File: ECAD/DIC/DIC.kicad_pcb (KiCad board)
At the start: 4 copper layers, 68.1 x 55.2 mm, 113 parts, among them J1 WE 62702621621, Q1 BC846, Q2 BC846, Q3 BC846, Q4 BC846, Q5 BC846, Q6 BC846, Q7 BC846, Q8 BC846, U1 R-78E5.0-1.0, U10 ADA4500-2, U2 MCP130-270, U3 STM32F072RBTx, U5 R-78E3.3-1.0, U7 MCP2562-E-SN, U8 NCP1117-12, U9 ADA4500-2, Y1 WE830055951

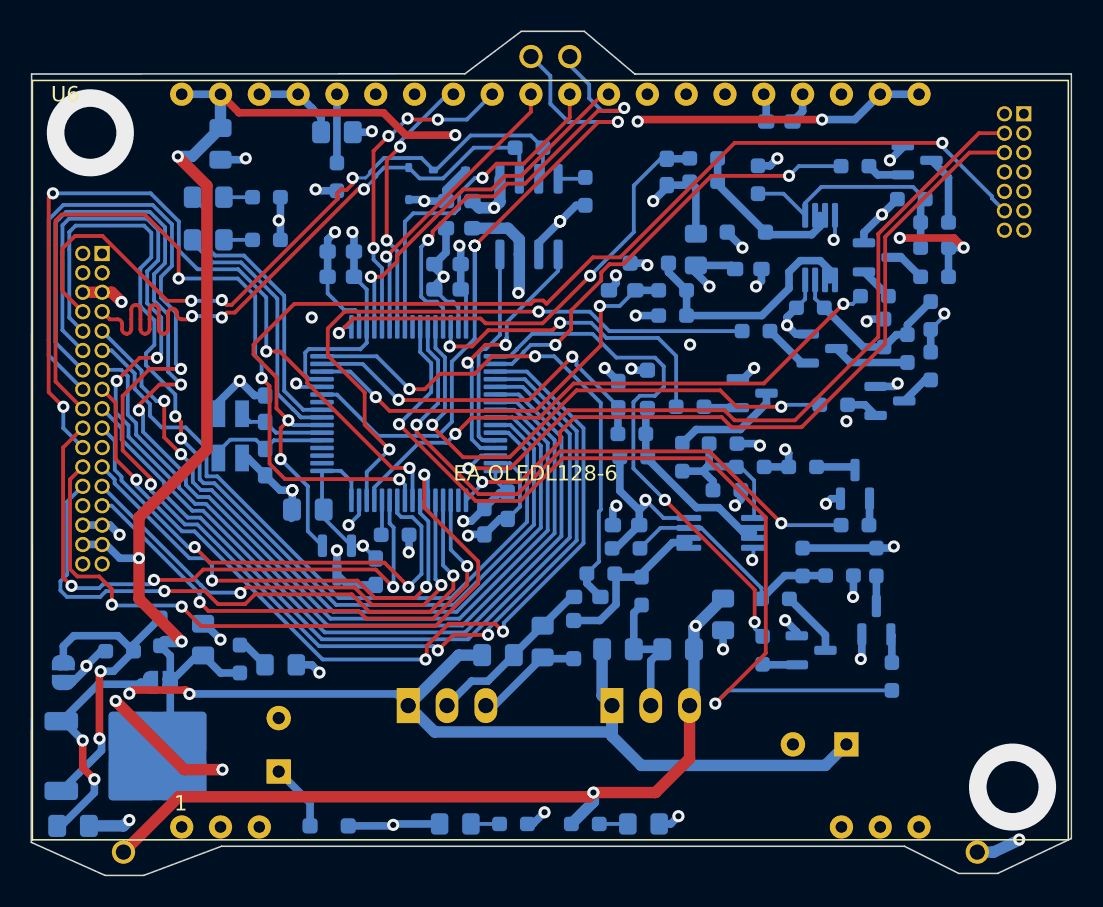
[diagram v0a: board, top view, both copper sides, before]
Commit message: finisjed PCB projekt
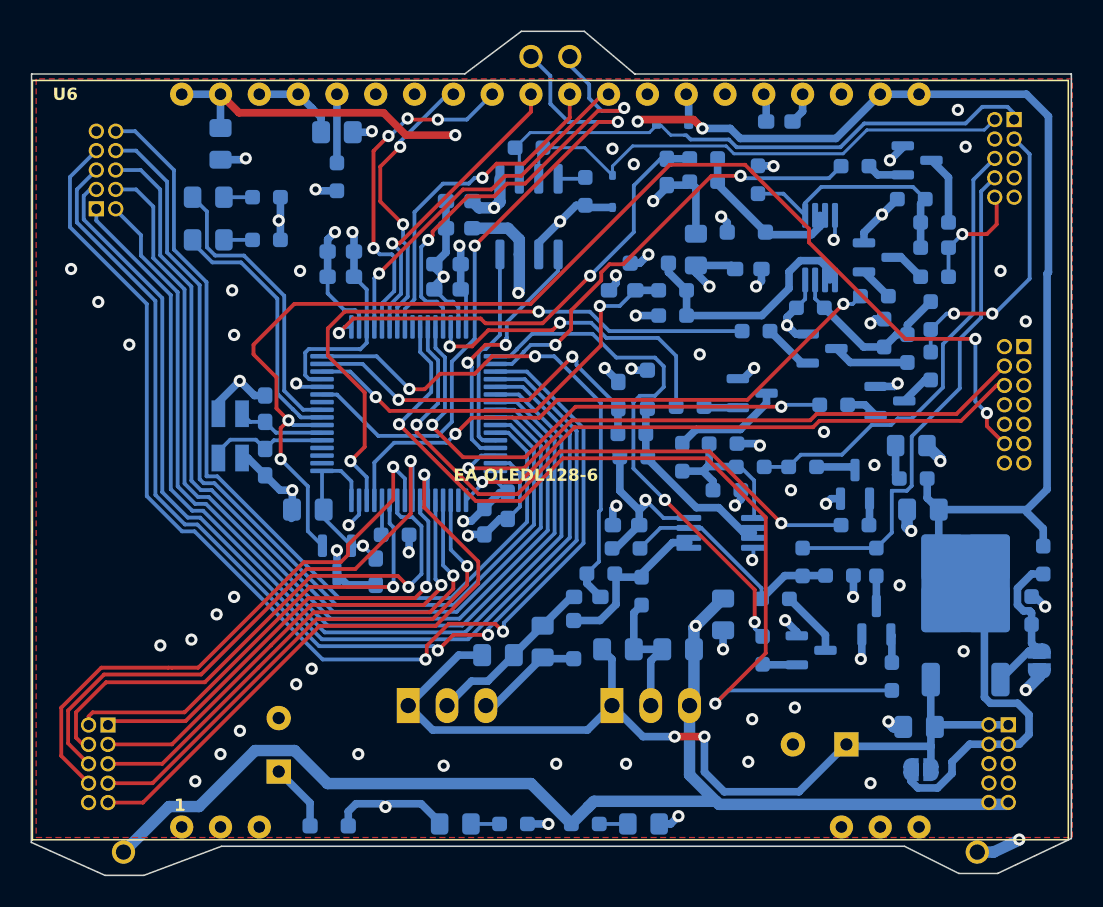
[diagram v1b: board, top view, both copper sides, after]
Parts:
- removed J1: WE 62702621621, Connector_PinHeader_1.27mm:PinHeader_2x17_P1.27mm_Vertical
- added J2: Conn_02x05_Top_Bottom, Connector_PinHeader_1.27mm:PinHeader_2x05_P1.27mm_Vertical, B.Cu at (76.2, 14.9)
- added J3: Conn_02x05_Top_Bottom, Connector_PinHeader_1.27mm:PinHeader_2x05_P1.27mm_Vertical, B.Cu at (75.8, 54.5)
- added J4: Conn_02x05_Top_Bottom, Connector_PinHeader_1.27mm:PinHeader_2x05_P1.27mm_Vertical, B.Cu at (16.1, 20.7)
- added J5: Conn_02x05_Top_Bottom, Connector_PinHeader_1.27mm:PinHeader_2x05_P1.27mm_Vertical, B.Cu at (16.9, 54.5)
- moved JP1 63.9 mm to (77.9, 50.3)
- moved R5 59.7 mm to (77.3, 47.0), turned to -90 degrees
- moved R7 58.0 mm to (78.1, 43.7), turned to 90 degrees
- moved C22 55.7 mm to (70.0, 54.6), turned to 180 degrees
- moved U8 55.1 mm to (73.0, 46.5), turned to 90 degrees
- moved JP2 50.1 mm to (70.1, 57.4), turned to 0 degrees
- moved C23 47.9 mm to (70.2, 40.4), turned to 180 degrees
- moved R8 45.6 mm to (69.6, 38.4), turned to 0 degrees
- moved 12VGood 43.7 mm to (69.5, 36.2)
- moved D4 17.7 mm to (53.8, 15.2), turned to 0 degrees
- moved JTAG1 15.2 mm to (76.8, 29.7)
- moved D5 10.8 mm to (49.9, 19.6), turned to -90 degrees
- renumbered 12VGood1 to 12VGood, 3V3Good1 to 3V3Good, 5VGood1 to 5VGood, Error1 to Error, Heart1 to Heart
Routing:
- net Analog2_In: track 99.9 -> 32.9 mm, vias 1 -> 0
- net Analog3_In: track 65.1 -> 7.65 mm, vias 2 -> 1
- net +BATT: track 118.5 -> 61.7 mm, vias 5 -> 2
- net Analog0_In: track 71.8 -> 18.9 mm, vias 1 -> 2
- net Analog1_In: track 80.4 -> 30.3 mm, vias 1 -> 0
- net +3.3V: track 111.5 -> 63.7 mm, vias 18 -> 13
- net +5V: track 149.4 -> 191.0 mm, vias 8 -> 6
- net GPIO3_5VOut: track 92.1 -> 72.8 mm, vias 4 -> 2
- net GPIO2_12VOut: track 79.2 -> 61.8 mm, vias 2 -> 0
- net GPIO3_In: track 60.4 -> 77.6 mm, vias 3 -> 2
- net GPIO2_In: track 80.6 -> 64.4 mm, vias 2 -> 0
- net GPIO5_12VOut: track 54.0 -> 37.9 mm, vias 4 -> 1
- net GPIO3_12VOut: track 53.4 -> 68.9 mm
- net +12V: track 110.9 -> 125.6 mm, vias 6 -> 3
- net GPIO1_12VOut: track 45.9 -> 59.3 mm
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- added copper zone on In1.Cu, net +3.3V
- added copper zone on F.Cu, net GND
- added copper zone on In2.Cu, net GND
- removed copper zone on In2.Cu, net +3.3V
- removed copper zone on In1.Cu, net GND

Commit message: few small changes
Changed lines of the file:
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@@
       (drillshape 0)
       (scaleselection 1)
-      (outputdirectory "")
+      (outputdirectory "Gerber/")
     )
   )
@@
     (fp_line (start 1 0.6) (end -0.7 0.6)
       (stroke (width 0.1) (type solid)) (layer "B.Fab"))
-    (pad "1" smd roundrect (at -1.025 0 180) (size 1.15 1.4) (layers "B.Cu" "B.Paste" "B.Mask") (roundrect_rratio 0.217391)
+    (pad "1" smd roundrect (at -1.025 0 180) (size 1.15 1.4) (layers "B.Cu" "B.Paste" "B.Mask") (roundrect_rratio 0.2173913043)
       (net 1 "GND") (pinfunction "K") (pintype "passive"))
-    (pad "2" smd roundrect (at 1.025 0 180) (size 1.15 1.4) (layers "B.Cu" "B.Paste" "B.Mask") (roundrect_rratio 0.217391)
+    (pad "2" smd roundrect (at 1.025 0 180) (size 1.15 1.4) (layers "B.Cu" "B.Paste" "B.Mask") (roundrect_rratio 0.2173913043)
       (net 14 "Net-(12VGood1-A)") (pinfunction "A") (pintype "passive"))
     (model "${KICAD6_3DMODEL_DIR}/LED_SMD.3dshapes/LED_0805_2012Metric.wrl"
@@
     (fp_line (start 1 0.625) (end 1 -0.625)
       (stroke (width 0.1) (type solid)) (layer "B.Fab"))
-    (pad "1" smd roundrect (at -1.0375 0 180) (size 1.175 1.45) (layers "B.Cu" "B.Paste" "B.Mask") (roundrect_rratio 0.212766)
+    (pad "1" smd roundrect (at -1.0375 0 180) (size 1.175 1.45) (layers "B.Cu" "B.Paste" "B.Mask") (roundrect_rratio 0.2127659574)
       (net 25 "+12V") (pintype "passive"))
-    (pad "2" smd roundrect (at 1.0375 0 180) (size 1.175 1.45) (layers "B.Cu" "B.Paste" "B.Mask") (roundrect_rratio 0.212766)
+    (pad "2" smd roundrect (at 1.0375 0 180) (size 1.175 1.45) (layers "B.Cu" "B.Paste" "B.Mask") (roundrect_rratio 0.2127659574)
       (net 1 "GND") (pintype "passive"))
     (model "${KICAD6_3DMODEL_DIR}/Capacitor_SMD.3dshapes/C_0805_2012Metric.wrl"
@@
     (fp_line (start 1 0.625) (end 1 -0.625)
       (stroke (width 0.1) (type solid)) (layer "B.Fab"))
-    (pad "1" smd roundrect (at -1.0375 0 180) (size 1.175 1.45) (layers "B.Cu" "B.Paste" "B.Mask") (roundrect_rratio 0.212766)
+    (pad "1" smd roundrect (at -1.0375 0 180) (size 1.175 1.45) (layers "B.Cu" "B.Paste" "B.Mask") (roundrect_rratio 0.2127659574)
       (net 7 "+BATT") (pintype "passive"))
-    (pad "2" smd roundrect (at 1.0375 0 180) (size 1.175 1.45) (layers "B.Cu" "B.Paste" "B.Mask") (roundrect_rratio 0.212766)
+    (pad "2" smd roundrect (at 1.0375 0 180) (size 1.175 1.45) (layers "B.Cu" "B.Paste" "B.Mask") (roundrect_rratio 0.2127659574)
       (net 1 "GND") (pintype "passive"))
     (model "${KICAD6_3DMODEL_DIR}/Capacitor_SMD.3dshapes/C_0805_2012Metric.wrl"
@@
     (fp_line (start 4.11 2.7) (end 4.11 -2.7)
       (stroke (width 0.1) (type solid)) (layer "B.Fab"))
-    (pad "1" smd roundrect (at -5.04 2.28 90) (size 2.2 1.2) (layers "B.Cu" "B.Paste" "B.Mask") (roundrect_rratio 0.208333)
+    (pad "1" smd roundrect (at -5.04 2.28 90) (size 2.2 1.2) (layers "B.Cu" "B.Paste" "B.Mask") (roundrect_rratio 0.2083333333)
       (net 59 "Net-(JP1-B)") (pinfunction "GND") (pintype "power_in"))
-    (pad "2" smd roundrect (at -0.415 -1.525 90) (size 3.05 2.75) (layers "B.Cu" "B.Paste") (roundrect_rratio 0.090909)
+    (pad "2" smd roundrect (at -0.415 -1.525 90) (size 3.05 2.75) (layers "B.Cu" "B.Paste") (roundrect_rratio 0.09090909091)
       (net 25 "+12V") (pinfunction "VO") (pintype "power_out"))
-    (pad "2" smd roundrect (at -0.415 1.525 90) (size 3.05 2.75) (layers "B.Cu" "B.Paste") (roundrect_rratio 0.090909)
+    (pad "2" smd roundrect (at -0.415 1.525 90) (size 3.05 2.75) (layers "B.Cu" "B.Paste") (roundrect_rratio 0.09090909091)
       (net 25 "+12V") (pinfunction "VO") (pintype "power_out"))
-    (pad "2" smd roundrect (at 1.26 0 90) (size 6.4 5.8) (layers "B.Cu" "B.Mask") (roundrect_rratio 0.043103)
+    (pad "2" smd roundrect (at 1.26 0 90) (size 6.4 5.8) (layers "B.Cu" "B.Mask") (roundrect_rratio 0.04310293103)
       (net 25 "+12V") (pinfunction "VO") (pintype "power_out"))
-    (pad "2" smd roundrect (at 2.935 -1.525 90) (size 3.05 2.75) (layers "B.Cu" "B.Paste") (roundrect_rratio 0.090909)
+    (pad "2" smd roundrect (at 2.935 -1.525 90) (size 3.05 2.75) (layers "B.Cu" "B.Paste") (roundrect_rratio 0.09090909091)
       (net 25 "+12V") (pinfunction "VO") (pintype "power_out"))
-    (pad "2" smd roundrect (at 2.935 1.525 90) (size 3.05 2.75) (layers "B.Cu" "B.Paste") (roundrect_rratio 0.090909)
+    (pad "2" smd roundrect (at 2.935 1.525 90) (size 3.05 2.75) (layers "B.Cu" "B.Paste") (roundrect_rratio 0.09090909091)
       (net 25 "+12V") (pinfunction "VO") (pintype "power_out"))
-    (pad "3" smd roundrect (at -5.04 -2.28 90) (size 2.2 1.2) (layers "B.Cu" "B.Paste" "B.Mask") (roundrect_rratio 0.208333)
+    (pad "3" smd roundrect (at -5.04 -2.28 90) (size 2.2 1.2) (layers "B.Cu" "B.Paste" "B.Mask") (roundrect_rratio 0.2083333333)
       (net 7 "+BATT") (pinfunction "VI") (pintype "power_in"))
     (model "${KICAD6_3DMODEL_DIR}/Package_TO_SOT_SMD.3dshapes/TO-252-2.wrl"
@@
     (fp_line (start 1 0.625) (end 1 -0.625)
       (stroke (width 0.1) (type solid)) (layer "B.Fab"))
-    (pad "1" smd roundrect (at -1.0375 0 270) (size 1.175 1.45) (layers "B.Cu" "B.Paste" "B.Mask") (roundrect_rratio 0.212766)
+    (pad "1" smd roundrect (at -1.0375 0 270) (size 1.175 1.45) (layers "B.Cu" "B.Paste" "B.Mask") (roundrect_rratio 0.2127659574)
       (net 8 "+5V") (pintype "passive"))
-    (pad "2" smd roundrect (at 1.0375 0 270) (size 1.175 1.45) (layers "B.Cu" "B.Paste" "B.Mask") (roundrect_rratio 0.212766)
+    (pad "2" smd roundrect (at 1.0375 0 270) (size 1.175 1.45) (layers "B.Cu" "B.Paste" "B.Mask") (roundrect_rratio 0.2127659574)
       (net 1 "GND") (pintype "passive"))
     (model "${KICAD6_3DMODEL_DIR}/Capacitor_SMD.3dshapes/C_0805_2012Metric.wrl"
@@
     (fp_line (start 1 0.625) (end 1 -0.625)
       (stroke (width 0.1) (type solid)) (layer "B.Fab"))
-    (pad "1" smd roundrect (at -1.0375 0 270) (size 1.175 1.45) (layers "B.Cu" "B.Paste" "B.Mask") (roundrect_rratio 0.212766)
+    (pad "1" smd roundrect (at -1.0375 0 270) (size 1.175 1.45) (layers "B.Cu" "B.Paste" "B.Mask") (roundrect_rratio 0.2127659574)
       (net 1 "GND") (pintype "passive"))
-    (pad "2" smd roundrect (at 1.0375 0 270) (size 1.175 1.45) (layers "B.Cu" "B.Paste" "B.Mask") (roundrect_rratio 0.212766)
+    (pad "2" smd roundrect (at 1.0375 0 270) (size 1.175 1.45) (layers "B.Cu" "B.Paste" "B.Mask") (roundrect_rratio 0.2127659574)
       (net 8 "+5V") (pintype "passive"))
     (model "${KICAD6_3DMODEL_DIR}/Capacitor_SMD.3dshapes/C_0805_2012Metric.wrl"
